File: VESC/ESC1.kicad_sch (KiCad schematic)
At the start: 37 parts, among them Q1 SP40N03GNJ, Q10 SP40N03GNJ, Q17 SP40N03GNJ, Q18 SP40N03GNJ, Q5 SP40N03GNJ, Q9 SP40N03GNJ, U4 AT32F421G8U7, U8 NSG2065Q

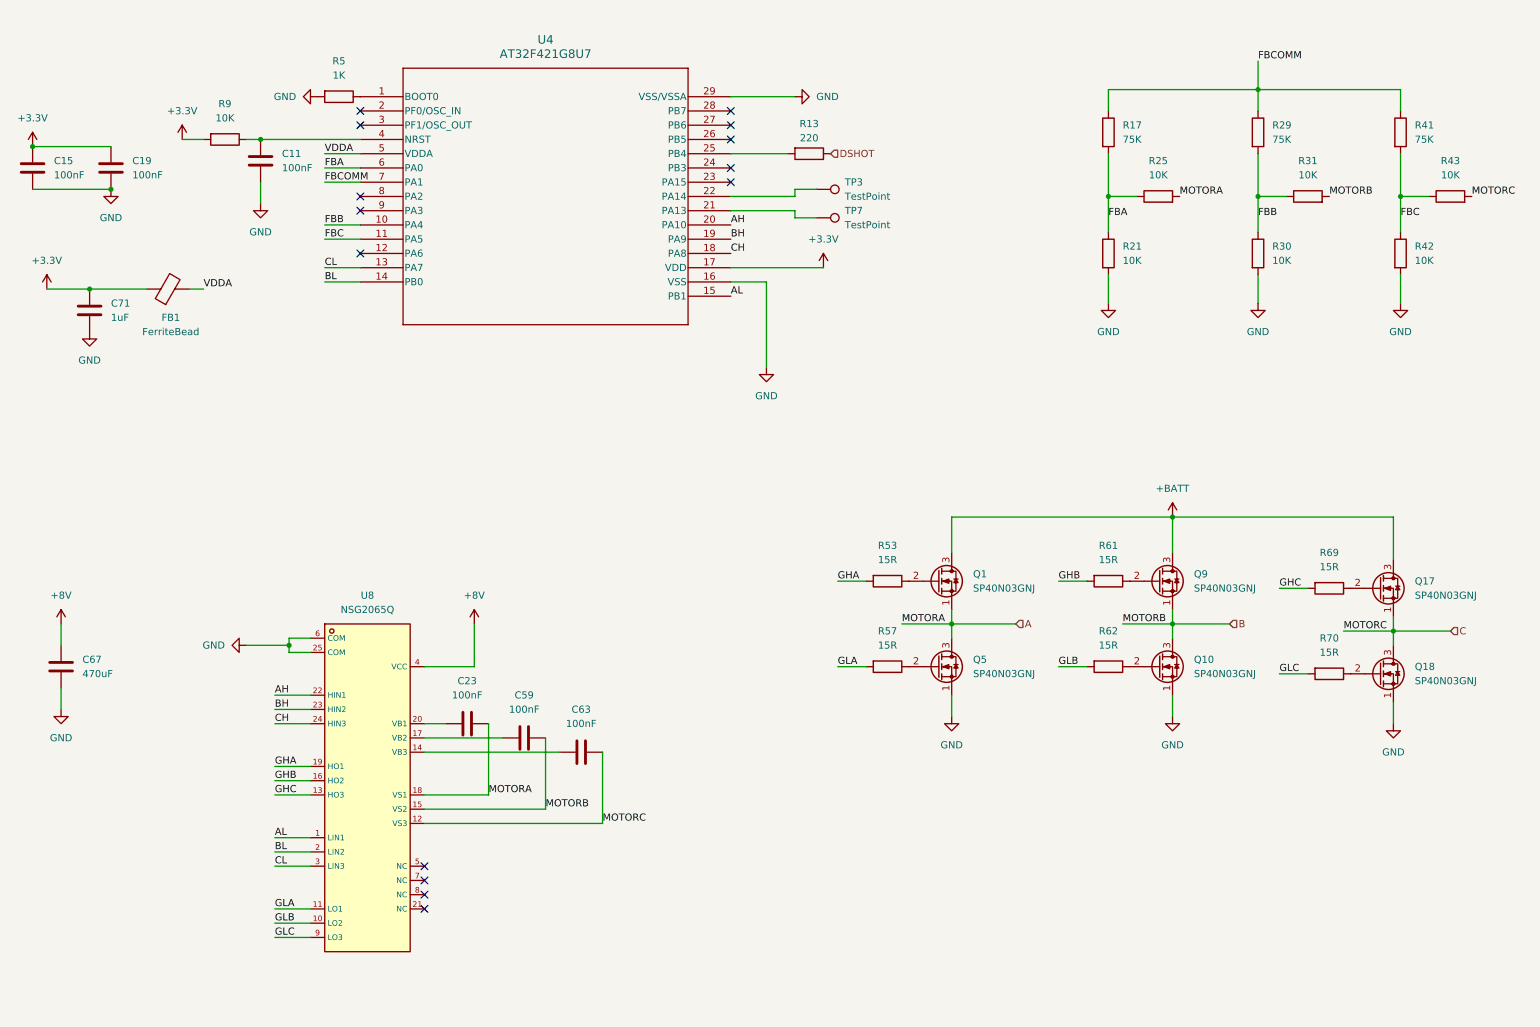
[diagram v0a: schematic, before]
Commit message: Revision_1 of VFC complete
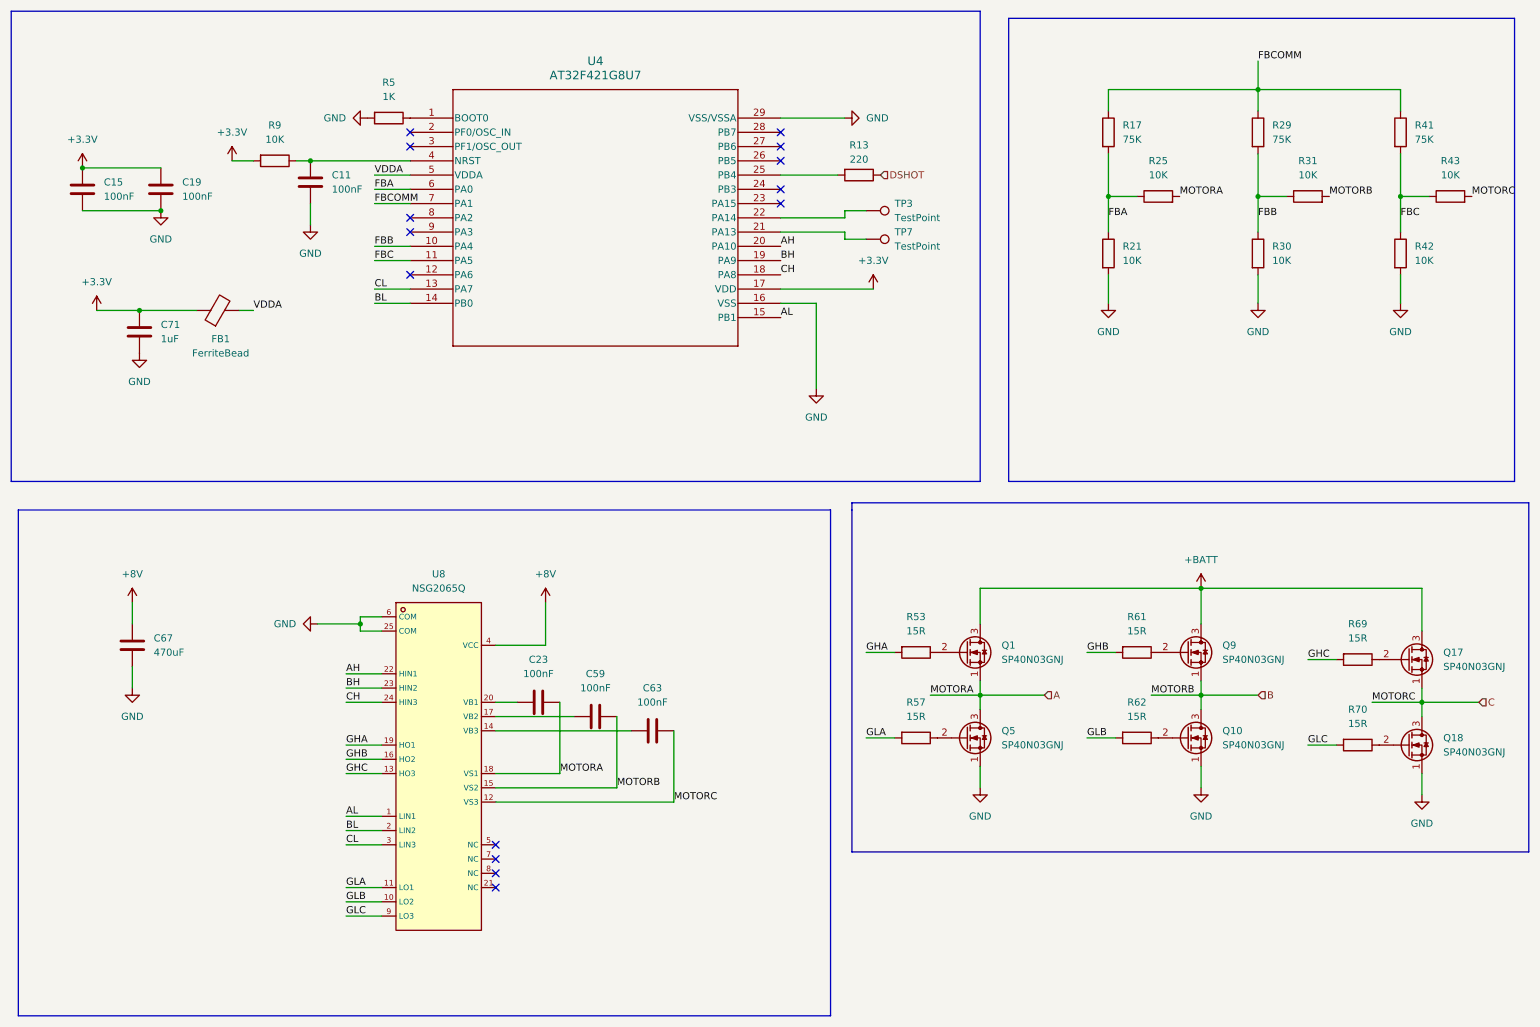
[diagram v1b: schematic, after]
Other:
- moved on the sheet: C11, C15, C19, C23, C59, C63, C67, C71, FB1, Q1, Q10, Q17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
